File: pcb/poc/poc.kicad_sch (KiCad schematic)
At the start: 19 parts, among them J1 MJ-4PP-9, SW00 EC_SW, SW01 EC_SW, SW10 EC_SW, SW11 EC_SW, U2 OPA350, U3 74HC4051

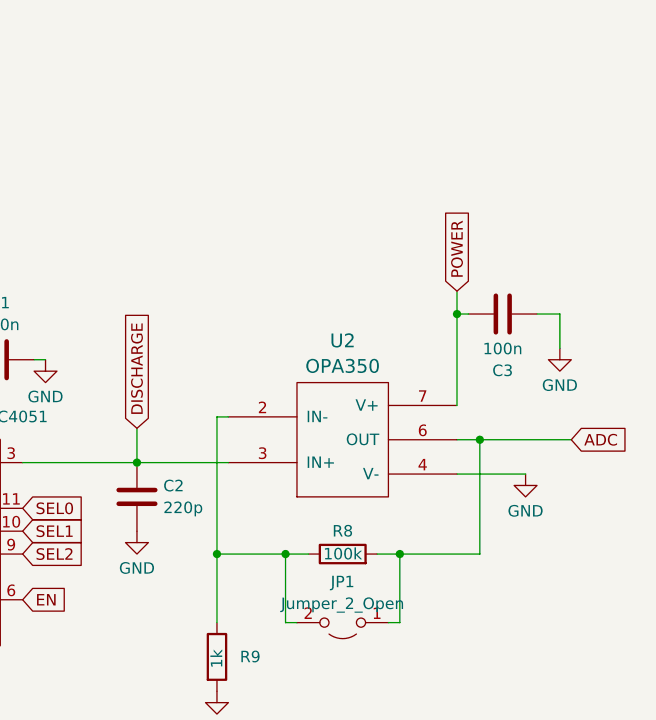
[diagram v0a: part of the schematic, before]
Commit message: release: sage60 v0.0.1
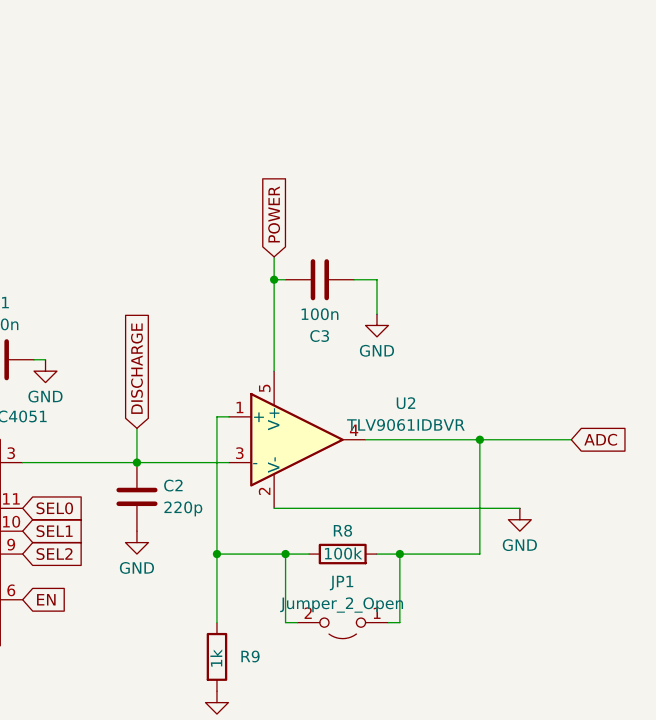
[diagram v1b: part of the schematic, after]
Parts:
- removed U2: OPA350, Package_SO:SOIC-8_3.9x4.9mm_P1.27mm, symbol 0_tako:OPA350
- added U2: TLV9061IDBVR, Package_TO_SOT_SMD:SOT-23-5, symbol Amplifier_Operational:TLV9001IDCK
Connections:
- net ADC: now also U2.4
- net DISCHARGE: now also U2.3 (-)
- net GND: now also U2.2 (V-)
- net POWER: now also U2.5 (V+)
- net at JP1.2 (B), R8.1, R9.1: now also U2.1 (+)
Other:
- moved on the sheet: C3
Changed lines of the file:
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@@
   (junction (at 88.9 130.81) (diameter 0) (color 0 0 0 0)
   )
-  (junction (at 157.48 96.52) (diameter 0) (color 0 0 0 0)
+  (junction (at 137.16 92.71) (diameter 0) (color 0 0 0 0)
   )
   (junction (at 49.53 77.47) (diameter 0) (color 0 0 0 0)
@@
     (stroke (width 0) (type default))
   )
-  (wire (pts (xy 160.02 110.49) (xy 157.48 110.49))
+  (wire (pts (xy 147.32 110.49) (xy 160.02 110.49))
     (stroke (width 0) (type default))
   )
@@
     (stroke (width 0) (type default))
   )
-  (wire (pts (xy 165.1 114.3) (xy 157.48 114.3))
-    (stroke (width 0) (type default))
-  )
   (wire (pts (xy 74.93 91.44) (xy 60.96 91.44))
     (stroke (width 0) (type default))
@@
     (stroke (width 0) (type default))
   )
-  (wire (pts (xy 157.48 96.52) (xy 157.48 106.68))
+  (wire (pts (xy 137.16 92.71) (xy 137.16 102.87))
     (stroke (width 0) (type default))
   )
@@
     (stroke (width 0) (type default))
   )
-  (wire (pts (xy 157.48 93.98) (xy 157.48 96.52))
+  (wire (pts (xy 137.16 90.17) (xy 137.16 92.71))
     (stroke (width 0) (type default))
   )
@@
     (stroke (width 0) (type default))
   )
-  (wire (pts (xy 168.91 96.52) (xy 166.37 96.52))
+  (wire (pts (xy 148.59 92.71) (xy 146.05 92.71))
     (stroke (width 0) (type default))
   )
@@
     (stroke (width 0) (type default))
   )
-  (wire (pts (xy 157.48 96.52) (xy 158.75 96.52))
+  (wire (pts (xy 137.16 92.71) (xy 138.43 92.71))
     (stroke (width 0) (type default))
   )
@@
     (stroke (width 0) (type default))
   )
-  (wire (pts (xy 168.91 100.33) (xy 168.91 96.52))
+  (wire (pts (xy 148.59 96.52) (xy 148.59 92.71))
     (stroke (width 0) (type default))
   )
@@
   )
   (wire (pts (xy 138.43 130.81) (xy 138.43 123.19))
+    (stroke (width 0) (type default))
+  )
+  (wire (pts (xy 137.16 118.11) (xy 164.465 118.11))
     (stroke (width 0) (type default))
   )
@@
     )
   )
-  (global_label "POWER" (shape input) (at 157.48 93.98 90) (fields_autoplaced)
-    (effects (font (size 1.27 1.27)) (justify left))
-    (property "Intersheetrefs" "${INTERSHEET_REFS}" (at 157.48 84.5239 90)
+  (global_label "POWER" (shape input) (at 137.16 90.17 90) (fields_autoplaced)
+    (effects (font (size 1.27 1.27)) (justify left))
+    (property "Intersheetrefs" "${INTERSHEET_REFS}" (at 137.16 80.7139 90)
       (effects (font (size 1.27 1.27)) (justify left) hide)
     )
@@
     )
   )
-  (symbol (lib_id "power:GND") (at 168.91 100.33 0) (unit 1)
-    (in_bom yes) (on_board yes) (dnp no) (fields_autoplaced)
-    (property "Reference" "#PWR06" (at 168.91 106.68 0)
-      (effects (font (size 1.27 1.27)) hide)
-    )
-    (property "Value" "GND" (at 168.91 104.4631 0)
-      (effects (font (size 1.27 1.27)))
-    )
-    (property "Footprint" "" (at 168.91 100.33 0)
-      (effects (font (size 1.27 1.27)) hide)
-    )
-    (property "Datasheet" "" (at 168.91 100.33 0)
+  (symbol (lib_id "power:GND") (at 148.59 96.52 0) (unit 1)
+    (in_bom yes) (on_board yes) (dnp no) (fields_autoplaced)
+    (property "Reference" "#PWR06" (at 148.59 102.87 0)
+      (effects (font (size 1.27 1.27)) hide)
+    )
+    (property "Value" "GND" (at 148.59 100.6531 0)
+      (effects (font (size 1.27 1.27)))
+    )
+    (property "Footprint" "" (at 148.59 96.52 0)
+      (effects (font (size 1.27 1.27)) hide)
+    )
+    (property "Datasheet" "" (at 148.59 96.52 0)
       (effects (font (size 1.27 1.27)) hide)
     )
@@
     )
   )
-  (symbol (lib_id "Device:C") (at 162.56 96.52 270) (unit 1)
-    (in_bom yes) (on_board yes) (dnp no) (fields_autoplaced)
-    (property "Reference" "C3" (at 162.56 102.8233 90)
-      (effects (font (size 1.27 1.27)))
-    )
-    (property "Value" "100n" (at 162.56 100.3991 90)
-      (effects (font (size 1.27 1.27)))
-    )
-    (property "Footprint" "Capacitor_SMD:C_0805_2012Metric_Pad1.18x1.45mm_HandSolder" (at 158.75 97.4852 0)
-      (effects (font (size 1.27 1.27)) hide)
-    )
-    (property "Datasheet" "~" (at 162.56 96.52 0)
+  (symbol (lib_id "Device:C") (at 142.24 92.71 270) (unit 1)
+    (in_bom yes) (on_board yes) (dnp no) (fields_autoplaced)
+    (property "Reference" "C3" (at 142.24 99.0133 90)
+      (effects (font (size 1.27 1.27)))
+    )
+    (property "Value" "100n" (at 142.24 96.5891 90)
+      (effects (font (size 1.27 1.27)))
+    )
+    (property "Footprint" "Capacitor_SMD:C_0805_2012Metric_Pad1.18x1.45mm_HandSolder" (at 138.43 93.6752 0)
+      (effects (font (size 1.27 1.27)) hide)
+    )
+    (property "Datasheet" "~" (at 142.24 92.71 0)
       (effects (font (size 1.27 1.27)) hide)
     )
@@
     )
   )
-  (symbol (lib_id "power:GND") (at 165.1 114.3 0) (unit 1)
+  (symbol (lib_id "power:GND") (at 164.465 118.11 0) (unit 1)
     (in_bom yes) (on_board yes) (dnp no)
-    (property "Reference" "#PWR07" (at 165.1 120.65 0)
-      (effects (font (size 1.27 1.27)) hide)
-    )
-    (property "Value" "GND" (at 165.1 118.4331 0)
-      (effects (font (size 1.27 1.27)))
-    )
-    (property "Footprint" "" (at 165.1 114.3 0)
-      (effects (font (size 1.27 1.27)) hide)
-    )
-    (property "Datasheet" "" (at 165.1 114.3 0)
+    (property "Reference" "#PWR07" (at 164.465 124.46 0)
+      (effects (font (size 1.27 1.27)) hide)
+    )
+    (property "Value" "GND" (at 164.465 122.2431 0)
+      (effects (font (size 1.27 1.27)))
+    )
+    (property "Footprint" "" (at 164.465 118.11 0)
+      (effects (font (size 1.27 1.27)) hide)
+    )
+    (property "Datasheet" "" (at 164.465 118.11 0)
       (effects (font (size 1.27 1.27)) hide)
     )
@@
         (path "/6e471c34-fb9c-4836-aac9-8239f9e8a673"
           (reference "R9") (unit 1)
+        )
+      )
+    )
+  )
+  (symbol (lib_id "Amplifier_Operational:TLV9001IDCK") (at 137.16 110.49 0) (unit 1)
+    (in_bom yes) (on_board yes) (dnp no) (fields_autoplaced)
+    (property "Reference" "U2" (at 151.8217 106.4728 0)
+      (effects (font (size 1.27 1.27)))
+    )
+    (property "Value" "TLV9061IDBVR" (at 151.8217 108.897 0)
+      (effects (font (size 1.27 1.27)))
+    )
+    (property "Footprint" "Package_TO_SOT_SMD:SOT-23-5" (at 142.24 110.49 0)
+      (effects (font (size 1.27 1.27)) hide)
+    )
+    (property "Datasheet" "https://datasheet.lcsc.com/lcsc/1912111437_Texas-Instruments-TLV9061IDBVR_C398358.pdf" (at 137.16 110.49 0)
+      (effects (font (size 1.27 1.27)) hide)
+    )
+    (pin "1")
+    (pin "2")
+    (pin "3")
+    (pin "4")
+    (pin "5")
+    (instances
+      (project "poc"
+        (path "/6e471c34-fb9c-4836-aac9-8239f9e8a673"
+          (reference "U2") (unit 1)
         )
       )
@@
         )
       )
-    )
-  )
-  (symbol (lib_id "0_tako:OPA350") (at 139.7 110.49 0) (unit 1)
-    (in_bom yes) (on_board yes) (dnp no)
-    (property "Reference" "U2" (at 144.78 99.5098 0)
-      (effects (font (size 1.524 1.524)))
-    )
-    (property "Value" "OPA350" (at 144.78 102.3426 0)
-      (effects (font (size 1.524 1.524)))
-    )
-    (property "Footprint" "Package_SO:SOIC-8_3.9x4.9mm_P1.27mm" (at 139.7 110.49 0)
-      (effects (font (size 1.524 1.524)) hide)
-    )
-    (property "Datasheet" "" (at 139.7 110.49 0)
-      (effects (font (size 1.524 1.524)))
-    )
-    (pin "2")
-    (pin "3")
-    (pin "4")
-    (pin "6")
-    (pin "7")
-    (instances
-      (project "poc"
-        (path "/6e471c34-fb9c-4836-aac9-8239f9e8a673"
-          (reference "U2") (unit 1)
-        )
-      )
